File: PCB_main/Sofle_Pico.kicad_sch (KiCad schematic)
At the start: 68 parts, among them J1 Conn_02x08_Top_Bottom, J2 Conn_02x08_Top_Bottom, J3 Conn_02x03, SW1 SW_PUSH, SW10 SW_PUSH, SW11 SW_PUSH, SW12 SW_PUSH, SW13 SW_PUSH, SW14 SW_PUSH, SW15 SW_PUSH, SW16 SW_PUSH, SW17 SW_PUSH, SW18 SW_PUSH, SW2 SW_PUSH, SW20 SW_PUSH, SW21 SW_PUSH, SW22 SW_PUSH, SW23 SW_PUSH, SW24 SW_PUSH, SW27 SW_PUSH, SW28 SW_PUSH, SW29 SW_PUSH, SW3 SW_PUSH, SW30 SW_PUSH, SW37 SW_PUSH, SW38 SW_PUSH, SW39 SW_PUSH, SW4 SW_PUSH, SW40 SW_PUSH, SW41 SW_PUSH, SW5 SW_PUSH, SW6 SW_PUSH, SW7 SW_PUSH, SW8 SW_PUSH, SW9 SW_PUSH, U2 Pico

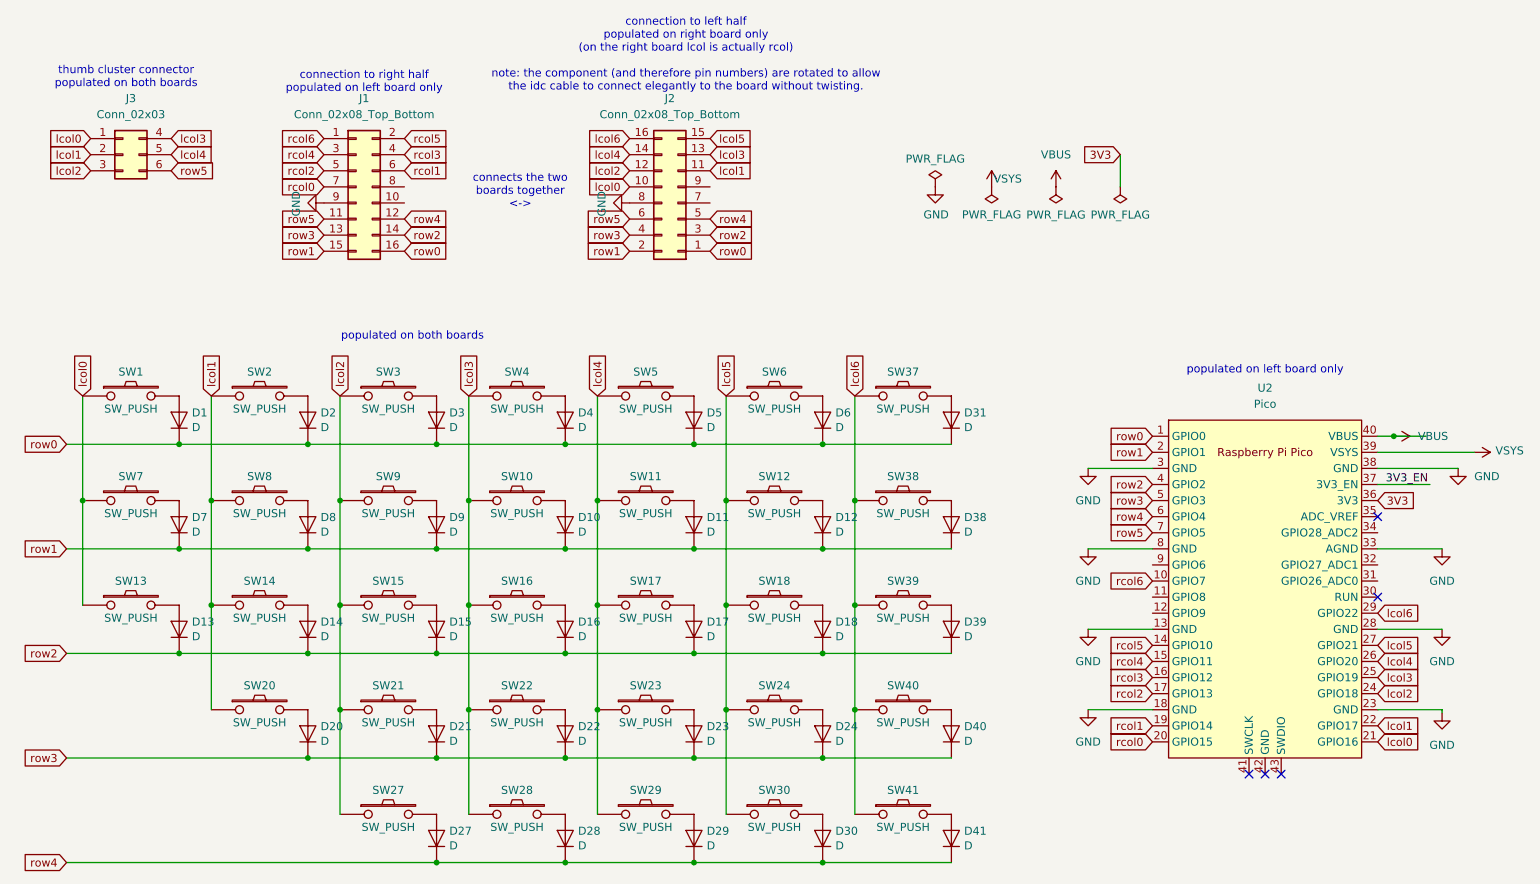
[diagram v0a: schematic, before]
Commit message: fix pcb
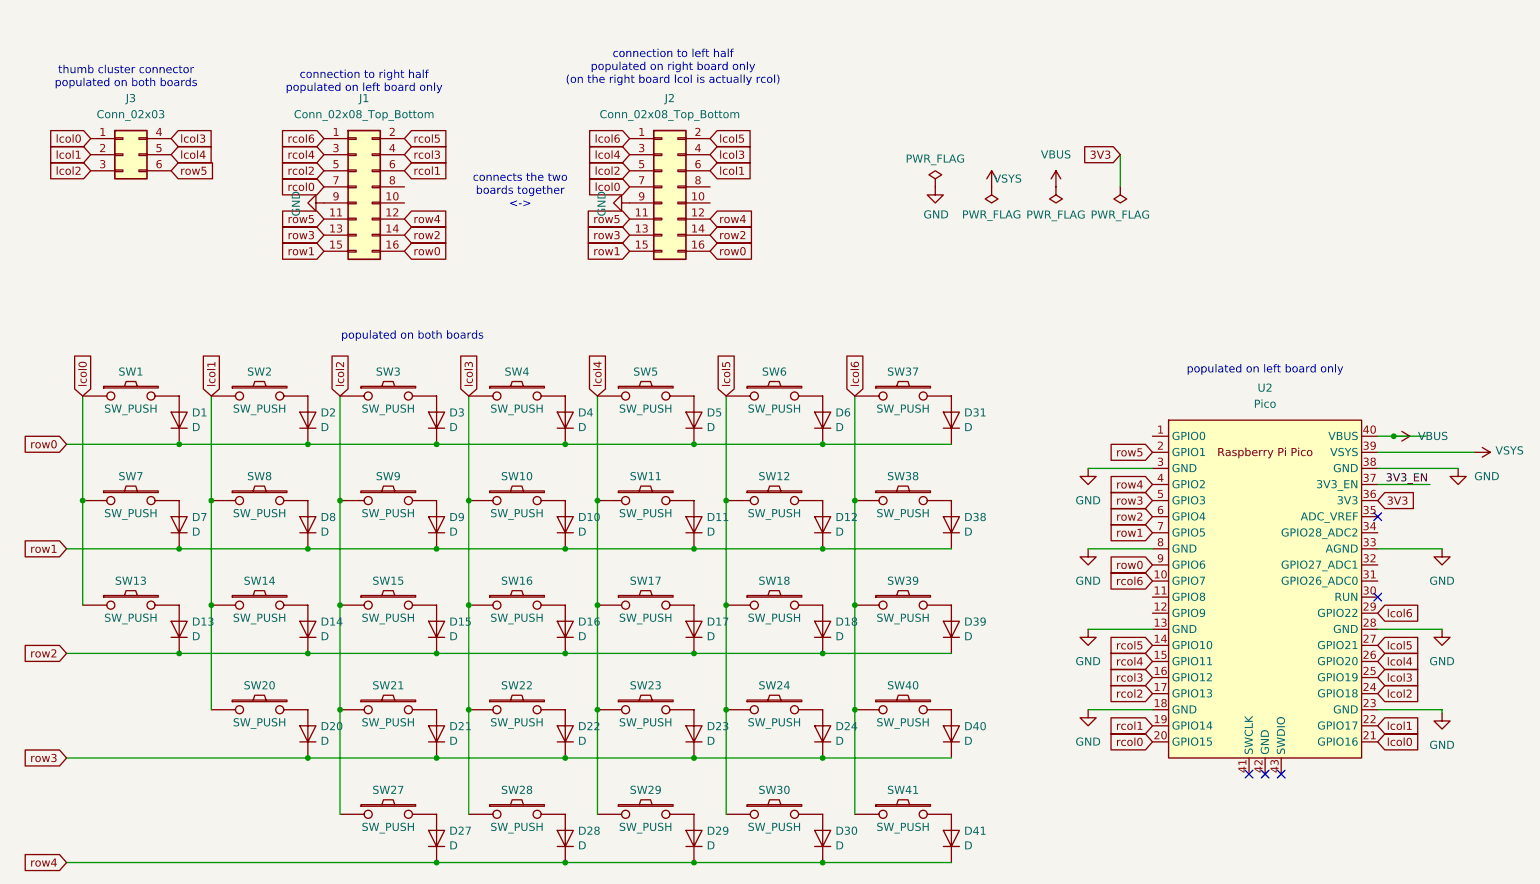
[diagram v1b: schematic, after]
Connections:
- net GND: now also J2.9 (Pin_9); no longer J2.8 (Pin_8)
- net lcol0: now also J2.7 (Pin_7); no longer J2.10 (Pin_10)
- net lcol1: now also J2.6 (Pin_6); no longer J2.11 (Pin_11)
- net lcol2: now also J2.5 (Pin_5); no longer J2.12 (Pin_12)
- net lcol3: now also J2.4 (Pin_4); no longer J2.13 (Pin_13)
- net lcol4: now also J2.3 (Pin_3); no longer J2.14 (Pin_14)
- net lcol5: now also J2.2 (Pin_2); no longer J2.15 (Pin_15)
- net lcol6: now also J2.1 (Pin_1); no longer J2.16 (Pin_16)
- net row0: now also J2.16 (Pin_16), U2.9 (GPIO6); no longer J2.1 (Pin_1), U2.1 (GPIO0)
- net row1: now also J2.15 (Pin_15), U2.7 (GPIO5); no longer J2.2 (Pin_2), U2.2 (GPIO1)
- net row2: now also J2.14 (Pin_14), U2.6 (GPIO4); no longer J2.3 (Pin_3), U2.4 (GPIO2)
- net row3: now also J2.13 (Pin_13); no longer J2.4 (Pin_4)
- net row4: now also J2.12 (Pin_12), U2.4 (GPIO2); no longer J2.5 (Pin_5), U2.6 (GPIO4)
- net row5: now also J2.11 (Pin_11), U2.2 (GPIO1); no longer J2.6 (Pin_6), U2.7 (GPIO5)
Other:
- note added: "connection to left half populated on right board only (on the right board lcol is actually rcol)"
- note removed: "connection to left half populated on right board only (on the right board lcol is actually rcol) note: the component (and therefore pin numbers) are rotated to allow the idc cable to connect elegantly to the board without twisting."
- moved on the sheet: J2
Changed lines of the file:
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@@
 		)
 	)
-	(text "connection to left half\npopulated on right board only\n(on the right board lcol is actually rcol)\n\nnote: the component (and therefore pin numbers) are rotated to allow\nthe idc cable to connect elegantly to the board without twisting."
+	(text "connection to left half\npopulated on right board only\n(on the right board lcol is actually rcol)"
 		(exclude_from_sim no)
-		(at 125.73 21.082 0)
+		(at 123.698 23.114 0)
 		(effects
 			(font
@@
 		)
 	)
-	(global_label "lcol5"
+	(global_label "row2"
 		(shape input)
-		(at 129.54 34.29 0)
+		(at 199.39 93.98 180)
+		(fields_autoplaced yes)
 		(effects
 			(font
 				(size 1.27 1.27)
 			)
-			(justify left)
+			(justify right)
 		)
 		(property "Intersheetrefs" "${INTERSHEET_REFS}"
-			(at 129.54 34.29 0)
+			(at 192.5838 93.98 0)
 			(effects
 				(font
 					(size 1.27 1.27)
 				)
-				(justify left)
+				(justify right)
 				(hide yes)
 			)
 		)
 	)
-	(global_label "row4"
+	(global_label "lcol5"
 		(shape input)
-		(at 199.39 93.98 180)
-		(fields_autoplaced yes)
+		(at 129.54 34.29 0)
 		(effects
 			(font
 				(size 1.27 1.27)
 			)
-			(justify right)
+			(justify left)
 		)
 		(property "Intersheetrefs" "${INTERSHEET_REFS}"
-			(at 192.5838 93.98 0)
+			(at 129.54 34.29 0)
 			(effects
 				(font
 					(size 1.27 1.27)
 				)
-				(justify right)
+				(justify left)
 				(hide yes)
 			)
@@
 		)
 	)
+	(global_label "row5"
+		(shape input)
+		(at 199.39 83.82 180)
+		(fields_autoplaced yes)
+		(effects
+			(font
+				(size 1.27 1.27)
+			)
+			(justify right)
+		)
+		(property "Intersheetrefs" "${INTERSHEET_REFS}"
+			(at 192.5838 83.82 0)
+			(effects
+				(font
+					(size 1.27 1.27)
+				)
+				(justify right)
+				(hide yes)
+			)
+		)
+	)
 	(global_label "row3"
 		(shape input)
@@
 		)
 	)
+	(global_label "row0"
+		(shape input)
+		(at 199.39 101.6 180)
+		(fields_autoplaced yes)
+		(effects
+			(font
+				(size 1.27 1.27)
+			)
+			(justify right)
+		)
+		(property "Intersheetrefs" "${INTERSHEET_REFS}"
+			(at 192.5838 101.6 0)
+			(effects
+				(font
+					(size 1.27 1.27)
+				)
+				(justify right)
+				(hide yes)
+			)
+		)
+	)
 	(global_label "row5"
 		(shape input)
@@
 		)
 	)
-	(global_label "row0"
-		(shape input)
-		(at 199.39 81.28 180)
-		(fields_autoplaced yes)
-		(effects
-			(font
-				(size 1.27 1.27)
-			)
-			(justify right)
-		)
-		(property "Intersheetrefs" "${INTERSHEET_REFS}"
-			(at 192.5838 81.28 0)
-			(effects
-				(font
-					(size 1.27 1.27)
-				)
-				(justify right)
-				(hide yes)
-			)
-		)
-	)
 	(global_label "lcol0"
 		(shape input)
@@
 		)
 	)
-	(global_label "row5"
+	(global_label "rcol5"
 		(shape input)
-		(at 199.39 96.52 180)
+		(at 199.39 114.3 180)
 		(fields_autoplaced yes)
 		(effects
@@
 		)
 		(property "Intersheetrefs" "${INTERSHEET_REFS}"
-			(at 192.5838 96.52 0)
+			(at 192.1605 114.3 0)
 			(effects
 				(font
@@
 		)
 	)
-	(global_label "rcol5"
+	(global_label "row1"
 		(shape input)
-		(at 199.39 114.3 180)
+		(at 199.39 96.52 180)
 		(fields_autoplaced yes)
 		(effects
@@
 		)
 		(property "Intersheetrefs" "${INTERSHEET_REFS}"
-			(at 192.1605 114.3 0)
+			(at 192.5838 96.52 0)
 			(effects
 				(font
@@
 	(global_label "row4"
 		(shape input)
-		(at 81.28 46.99 0)
+		(at 199.39 88.9 180)
 		(fields_autoplaced yes)
 		(effects
@@
 				(size 1.27 1.27)
 			)
-			(justify left)
-		)
-		(property "Intersheetrefs" "${INTERSHEET_REFS}"
-			(at 88.0862 46.99 0)
-			(effects
-				(font
-					(size 1.27 1.27)
-				)
-				(justify left)
-				(hide yes)
-			)
-		)
-	)
-	(global_label "row1"
-		(shape input)
-		(at 27.94 99.06 180)
-		(effects
-			(font
-				(size 1.27 1.27)
-			)
 			(justify right)
 		)
 		(property "Intersheetrefs" "${INTERSHEET_REFS}"
-			(at 27.94 99.06 0)
+			(at 192.5838 88.9 0)
 			(effects
 				(font
 					(size 1.27 1.27)
 				)
+				(justify right)
 				(hide yes)
 			)
 		)
 	)
-	(global_label "rcol1"
+	(global_label "row4"
 		(shape input)
-		(at 199.39 127 180)
+		(at 81.28 46.99 0)
 		(fields_autoplaced yes)
 		(effects
@@
 				(size 1.27 1.27)
 			)
-			(justify right)
+			(justify left)
 		)
 		(property "Intersheetrefs" "${INTERSHEET_REFS}"
-			(at 192.1605 127 0)
+			(at 88.0862 46.99 0)
 			(effects
 				(font
 					(size 1.27 1.27)
 				)
-				(justify right)
+				(justify left)
 				(hide yes)
 			)
 		)
 	)
-	(global_label "rcol4"
+	(global_label "row1"
 		(shape input)
-		(at 199.39 116.84 180)
-		(fields_autoplaced yes)
+		(at 27.94 99.06 180)
 		(effects
 			(font
@@
 		)
 		(property "Intersheetrefs" "${INTERSHEET_REFS}"
-			(at 192.1605 116.84 0)
+			(at 27.94 99.06 0)
 			(effects
 				(font
 					(size 1.27 1.27)
 				)
-				(justify right)
 				(hide yes)
 			)
 		)
 	)
-	(global_label "row1"
+	(global_label "rcol1"
 		(shape input)
-		(at 199.39 83.82 180)
+		(at 199.39 127 180)
 		(fields_autoplaced yes)
 		(effects
@@
 		)
 		(property "Intersheetrefs" "${INTERSHEET_REFS}"
-			(at 192.5838 83.82 0)
+			(at 192.1605 127 0)
 			(effects
 				(font
@@
 		)
 	)
-	(global_label "row2"
+	(global_label "rcol4"
 		(shape input)
-		(at 199.39 88.9 180)
+		(at 199.39 116.84 180)
 		(fields_autoplaced yes)
 		(effects
@@
 		)
 		(property "Intersheetrefs" "${INTERSHEET_REFS}"
-			(at 192.5838 88.9 0)
+			(at 192.1605 116.84 0)
 			(effects
 				(font
@@
 	(symbol
 		(lib_id "Connector_Generic:Conn_02x08_Odd_Even")
-		(at 124.46 44.45 180)
+		(at 121.92 41.91 0)
 		(unit 1)
 		(exclude_from_sim no)
@@
 		)
 		(property "Footprint" "Connector_PinHeader_2.00mm:PinHeader_2x08_P2.00mm_Vertical"
-			(at 124.46 44.45 0)
+			(at 121.92 41.91 0)
 			(effects
 				(font
@@
 		)
 		(property "Datasheet" "~"
-			(at 124.46 44.45 0)
+			(at 121.92 41.91 0)
 			(effects
 				(font
@@
 		)
 		(property "Description" "Generic connector, double row, 02x08, odd/even pin numbering scheme (row 1 odd numbers, row 2 even numbers), script generated (kicad-library-utils/schlib/autogen/connector/)"
-			(at 124.46 44.45 0)
+			(at 121.92 41.91 0)
 			(effects
 				(font
